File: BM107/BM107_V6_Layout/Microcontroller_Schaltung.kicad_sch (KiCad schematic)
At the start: 9 parts, among them J7 Sockel_BluePill, J8 Conn_01x02_Pin, U1 SN65HVD233, U2 LT1999-50

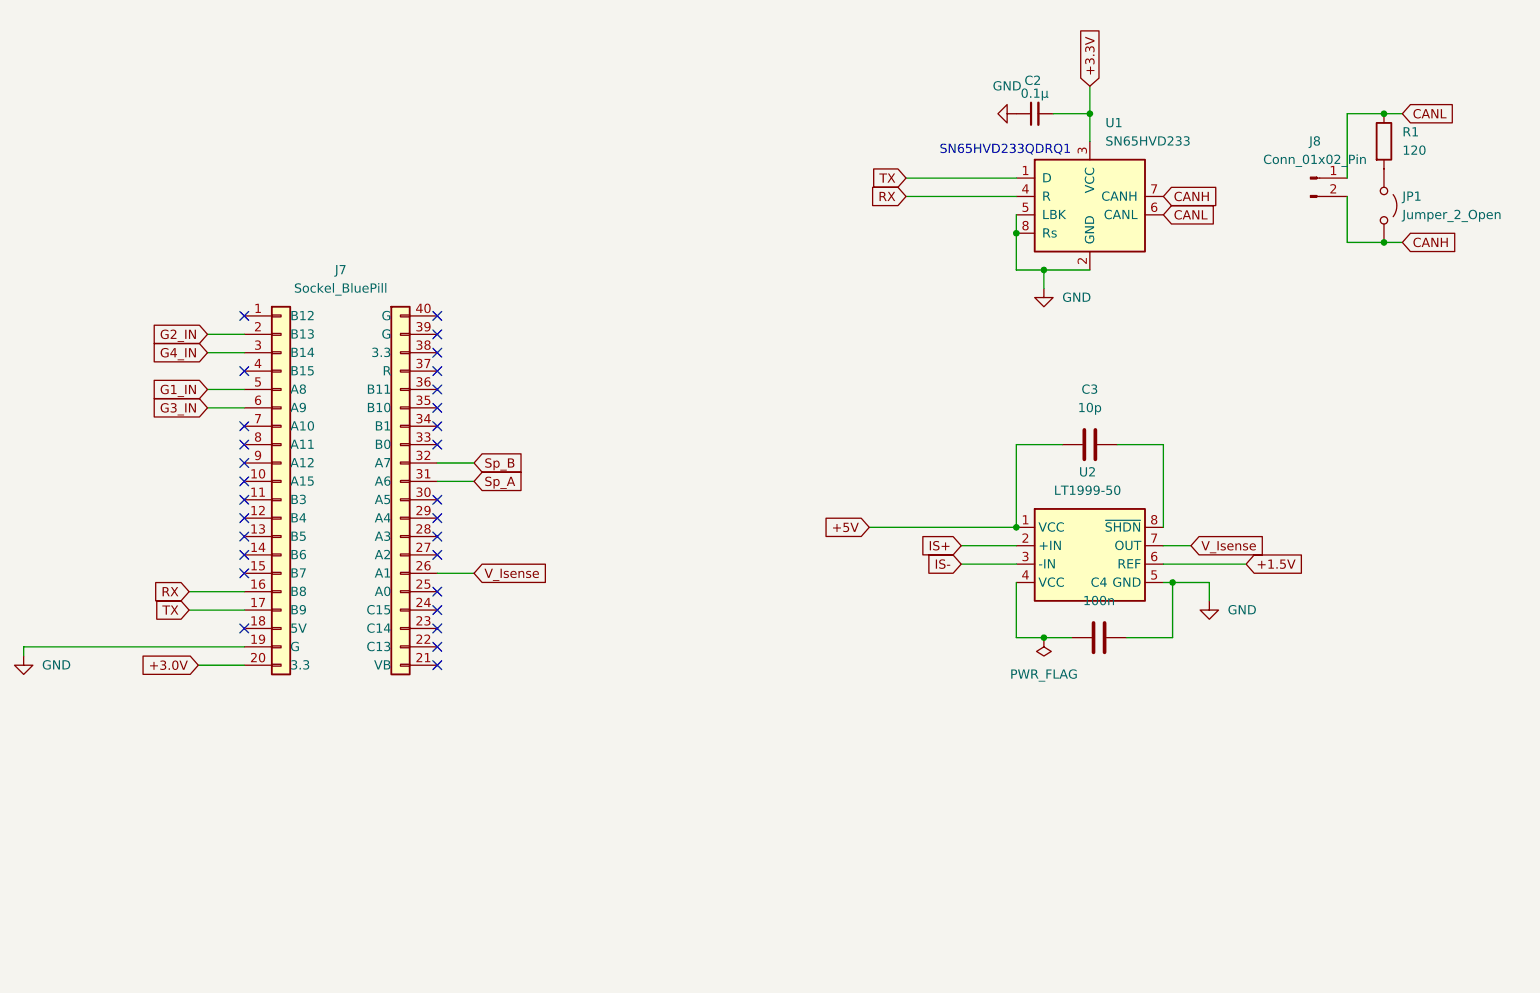
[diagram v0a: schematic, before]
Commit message: bm107 neu
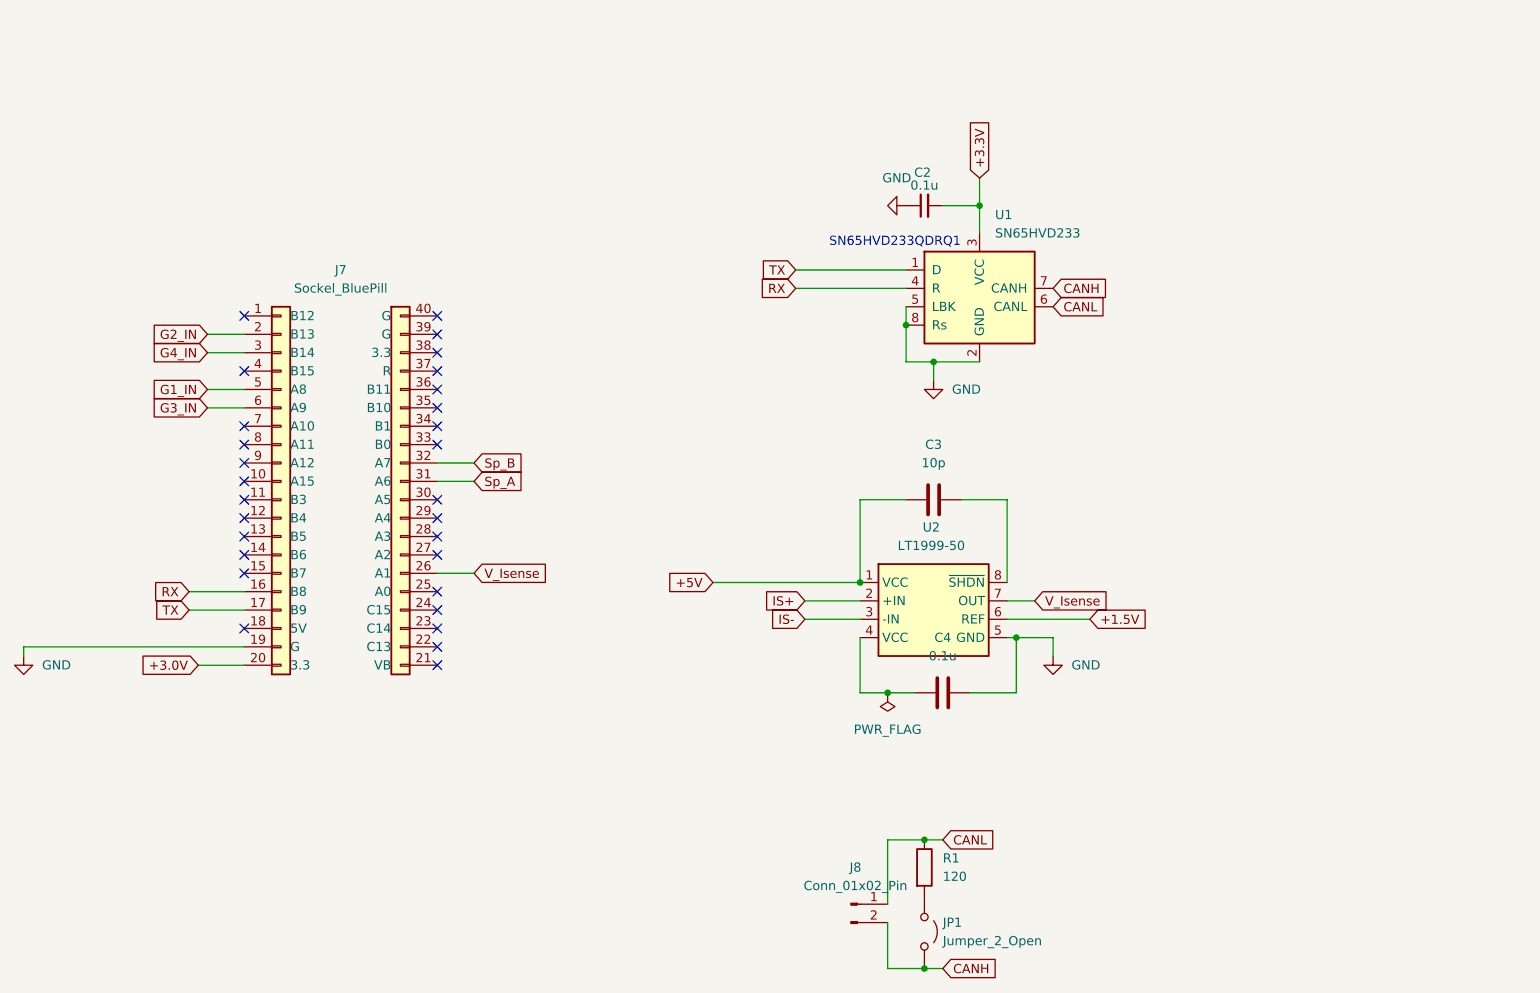
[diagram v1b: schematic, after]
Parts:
- C2: value 0.1µ -> 0.1u
- C4: value 100n -> 0.1u
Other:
- moved on the sheet: C2, C3, C4, J8, JP1, R1, U1, U2
